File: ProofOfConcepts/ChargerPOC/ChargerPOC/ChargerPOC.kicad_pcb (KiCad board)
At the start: 2 copper layers, 30 parts, among them J4 USB_C_Receptacle_USB2.0, U1 BSD316, U11 XL6009, U2 BSD316, U3 BSD316, U4 BSD316, U5 PC817, U6 PC817, U7 PC817, U8 PC817

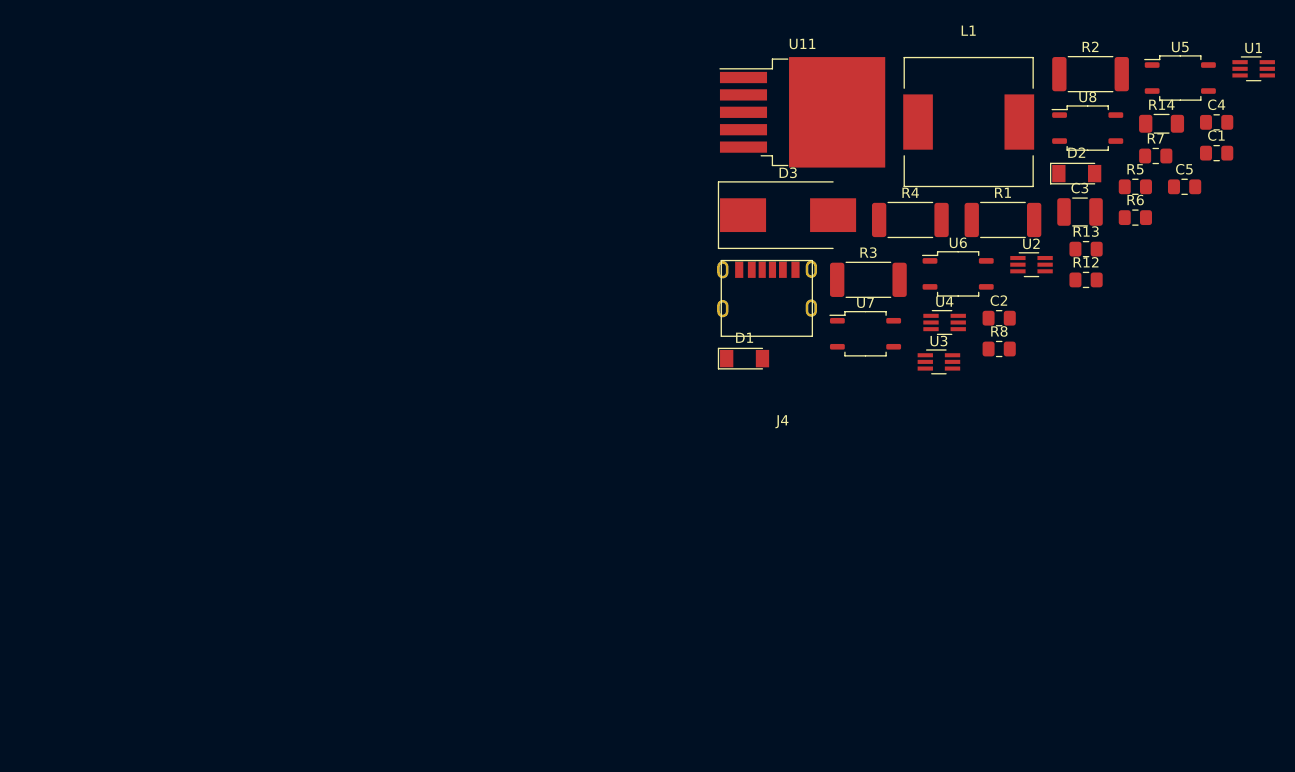
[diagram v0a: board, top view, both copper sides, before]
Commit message: E
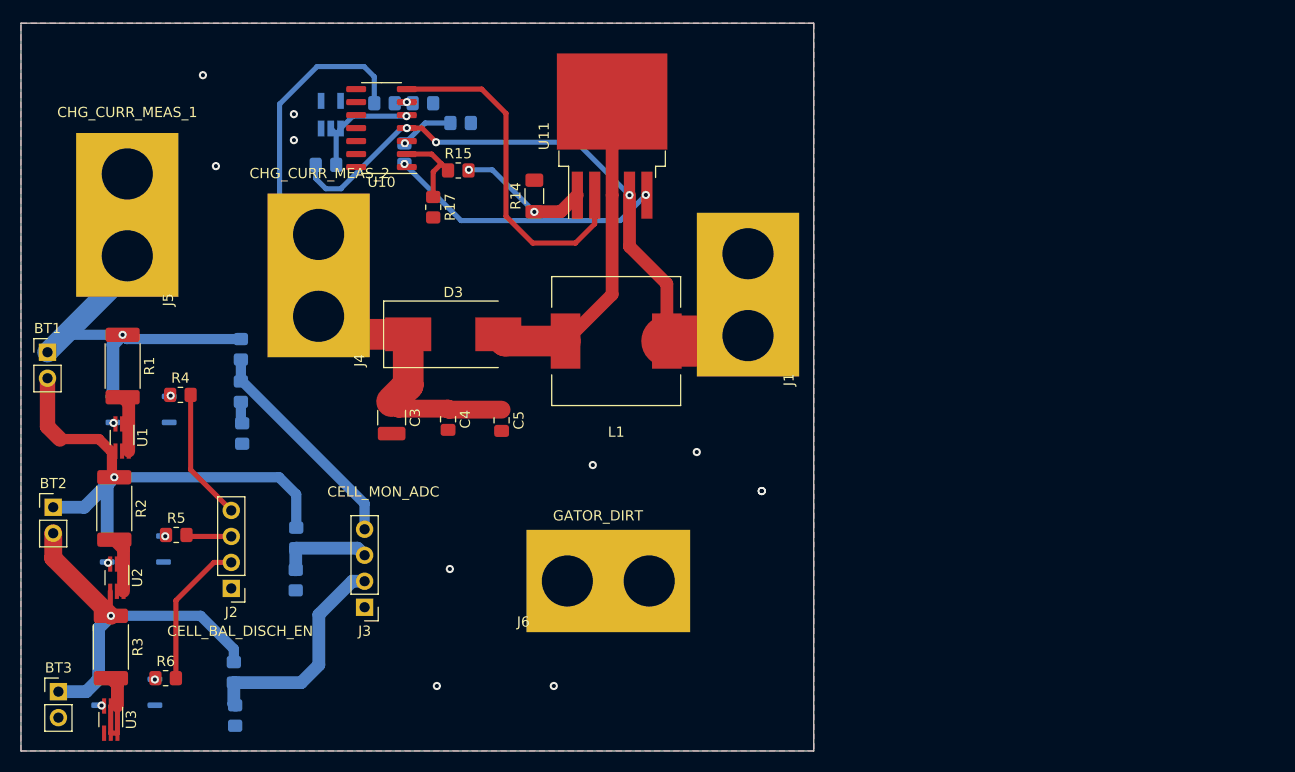
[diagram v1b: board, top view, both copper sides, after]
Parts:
- removed C1, C2: 10uF, Capacitor_SMD:C_0805_2012Metric_Pad1.18x1.45mm_HandSolder
- removed D1, D2: LL4148, Diode_SMD:D_MiniMELF
- removed R12, R13: 5.1k, Capacitor_SMD:C_0805_2012Metric_Pad1.18x1.45mm_HandSolder
- removed U7, U8: PC817, Package_SO:SOP-4_3.8x4.1mm_P2.54mm
- added BT1: Battery_Cell, Connector_PinHeader_2.54mm:PinHeader_1x02_P2.54mm_Vertical, F.Cu at (25.5, 91.8)
- added BT2: Battery_Cell, Connector_PinHeader_2.54mm:PinHeader_1x02_P2.54mm_Vertical, F.Cu at (26.0, 107.0)
- added BT3: Battery_Cell, Connector_PinHeader_2.54mm:PinHeader_1x02_P2.54mm_Vertical, F.Cu at (26.5, 125.0)
- added J1: VIN, 1KicadLib:GatorTestpoint, F.Cu at (92.6, 94.7)
- added J2: CELL_BAL_DISCH_EN, Connector_PinHeader_2.54mm:PinHeader_1x04_P2.54mm_Vertical, F.Cu at (43.4, 114.9)
- added J3: CELL_MON_ADC, Connector_PinHeader_2.54mm:PinHeader_1x04_P2.54mm_Vertical, F.Cu at (56.4, 116.8)
- added J5: CHG_CURR_MEAS_1, 1KicadLib:GatorTestpoint, F.Cu at (31.9, 86.9)
- added J6: GATOR_DIRT, 1KicadLib:GatorTestpoint, F.Cu at (71.8, 112.9)
- added R10: 18k, Resistor_SMD:R_0805_2012Metric_Pad1.20x1.40mm_HandSolder, B.Cu at (62.1, 67.5)
- added R11: 500, Resistor_SMD:R_0805_2012Metric_Pad1.20x1.40mm_HandSolder, B.Cu at (52.7, 73.5)
- added R15: 1k, Resistor_SMD:R_0805_2012Metric_Pad1.20x1.40mm_HandSolder, F.Cu at (65.6, 74.1)
- added R16: 1k, Resistor_SMD:R_0805_2012Metric_Pad1.20x1.40mm_HandSolder, B.Cu at (65.8, 69.4)
- added R17: 12.5k, Resistor_SMD:R_0805_2012Metric_Pad1.20x1.40mm_HandSolder, F.Cu at (63.1, 77.7)
- added R18: 12.5k, Resistor_SMD:R_0805_2012Metric_Pad1.20x1.40mm_HandSolder, B.Cu at (60.3, 72.4)
- added R19: 390, Resistor_SMD:R_0805_2012Metric_Pad1.20x1.40mm_HandSolder, B.Cu at (44.5, 99.8)
- added R20: 180k, Resistor_SMD:R_0805_2012Metric_Pad1.20x1.40mm_HandSolder, B.Cu at (49.8, 110.0)
- added R21: 68k, Resistor_SMD:R_0805_2012Metric_Pad1.20x1.40mm_HandSolder, B.Cu at (49.7, 114.1)
- added R22: 56k, Resistor_SMD:R_0805_2012Metric_Pad1.20x1.40mm_HandSolder, B.Cu at (43.7, 123.1)
- added R23: 68k, Resistor_SMD:R_0805_2012Metric_Pad1.20x1.40mm_HandSolder, B.Cu at (43.8, 127.3)
- added R9: 100k, Resistor_SMD:R_0805_2012Metric_Pad1.20x1.40mm_HandSolder, B.Cu at (58.4, 67.5)
- added U10: LM324, Package_SO:SOIC-14_3.9x8.7mm_P1.27mm, F.Cu at (58.1, 69.9)
- added U9: AS431, Package_TO_SOT_SMD:SOT-23-5_HandSoldering, B.Cu at (53.1, 68.6)
- J4: value USB_C_Receptacle_USB2.0 -> CHG_CURR_MEAS_2; footprint 1KicadLib:USB4125-GF-A -> 1KicadLib:GatorTestpoint
- R4: value 28.7 -> 200; footprint Resistor_SMD:R_2512_6332Metric_Pad1.40x3.35mm_HandSolder -> Resistor_SMD:R_0805_2012Metric_Pad1.20x1.40mm_HandSolder
- R5, R6: footprint Capacitor_SMD:C_0805_2012Metric_Pad1.18x1.45mm_HandSolder -> Resistor_SMD:R_0805_2012Metric_Pad1.20x1.40mm_HandSolder
- R7: value 200 -> 100k; footprint Capacitor_SMD:C_0805_2012Metric_Pad1.18x1.45mm_HandSolder -> Resistor_SMD:R_0805_2012Metric_Pad1.20x1.40mm_HandSolder; moved to B.Cu
- R8: value 200 -> 22k; footprint Capacitor_SMD:C_0805_2012Metric_Pad1.18x1.45mm_HandSolder -> Resistor_SMD:R_0805_2012Metric_Pad1.20x1.40mm_HandSolder; moved to B.Cu
- U4: value BSD316 -> PC817; footprint Package_TO_SOT_SMD:SOT-363_SC-70-6_Handsoldering -> Package_SO:SOP-4_3.8x4.1mm_P2.54mm; moved to B.Cu
- U5, U6: moved to B.Cu
- moved U1 116.3 mm to (32.7, 100.2), turned to -90 degrees
- moved U5 112.0 mm to (34.0, 111.1), turned to 180 degrees
- moved R6 104.9 mm to (37.0, 123.7)
- moved R2 104.4 mm to (32.0, 107.1), turned to -90 degrees
- moved R5 99.7 mm to (38.0, 109.7)
- moved U2 94.5 mm to (32.2, 113.9), turned to -90 degrees
- moved R7 91.4 mm to (44.3, 91.6), turned to -90 degrees
- moved U6 90.9 mm to (33.2, 125.1), turned to 180 degrees
- moved U3 88.2 mm to (31.6, 127.7), turned to -90 degrees
- moved R1 87.2 mm to (32.8, 93.2), turned to -90 degrees
- moved R3 82.3 mm to (31.6, 120.7), turned to -90 degrees
- moved C4 80.5 mm to (64.6, 98.4), turned to -90 degrees
- moved U4 79.0 mm to (34.6, 97.4), turned to 180 degrees
- moved R8 74.2 mm to (44.3, 95.7), turned to -90 degrees
- moved R4 73.3 mm to (38.4, 96.0)
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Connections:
- R1 pad 1: +BATT -> Net-(BT1-Pad1)
- R4 pad 1: Net-(BT3-Pad2) -> Net-(R4-Pad1)
- R4 pad 2: Net-(R4-Pad2) -> Net-(J2-Pad4)
- R7 pad 1: Net-(R7-Pad1) -> Net-(BT1-Pad1)
- R7 pad 2: Net-(J2-Pad3) (its old number) -> Net-(J3-Pad4)
- R8 pad 1: Net-(R8-Pad1) -> Net-(J3-Pad4)
- U3 pad 4: Net-(BT3-Pad2) -> GND
- U4 pad 1: Net-(R4-Pad2) -> Net-(R4-Pad1)
- U4 pad 2: Net-(R4-Pad2) -> GND
- U4 pad 3: Net-(U4-Pad3) -> Net-(U1-Pad3)
- U4 pad 4: GND -> Net-(BT1-Pad1)
- U5 pad 3: Net-(U1-Pad3) -> Net-(U2-Pad3)
- U5 pad 4: Vdrive -> Net-(BT1-Pad2)
- U6 pad 3: Net-(U2-Pad3) -> Net-(U3-Pad3)
- U6 pad 4: Vdrive -> Net-(BT2-Pad2)
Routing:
- net VBUS: track 0.00 -> 61.5 mm, vias 0 -> 3
- net +BATT: track 0.00 -> 55.9 mm
- net Net-(BT1-Pad2): track 0.00 -> 49.5 mm, vias 0 -> 1
- net Net-(BT1-Pad1): track 0.00 -> 38.8 mm, vias 0 -> 1
- net Net-(BT2-Pad2): track 0.00 -> 38.6 mm, vias 0 -> 1
- net Net-(U10-Pad7): track 0.00 -> 34.1 mm
- net Net-(D3-Pad2): track 0.00 -> 32.1 mm
- net Net-(R18-Pad2): track 0.00 -> 27.0 mm, vias 0 -> 2
- net Net-(J3-Pad2): track 0.00 -> 22.0 mm
- net Net-(J3-Pad4): track 0.00 -> 21.7 mm
- net Net-(J2-Pad2): track 0.00 -> 14.5 mm
- net Net-(R14-Pad1): track 0.00 -> 13.3 mm, vias 0 -> 2
- net Net-(J2-Pad4): track 0.00 -> 12.9 mm
- net Net-(R11-Pad2): track 0.00 -> 11.4 mm, vias 0 -> 1
- net Net-(R3-Pad2): track 0.00 -> 9.60 mm
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- added copper zone on B.Cu, net GND
- added copper zone on F.Cu, net GND
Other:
- board outline added: 77.5 x 71.1 mm
